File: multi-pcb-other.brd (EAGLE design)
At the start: 83.8 x 33 mm, 7 parts, among them X1 8B-ZR, X2 2.52B-ZR

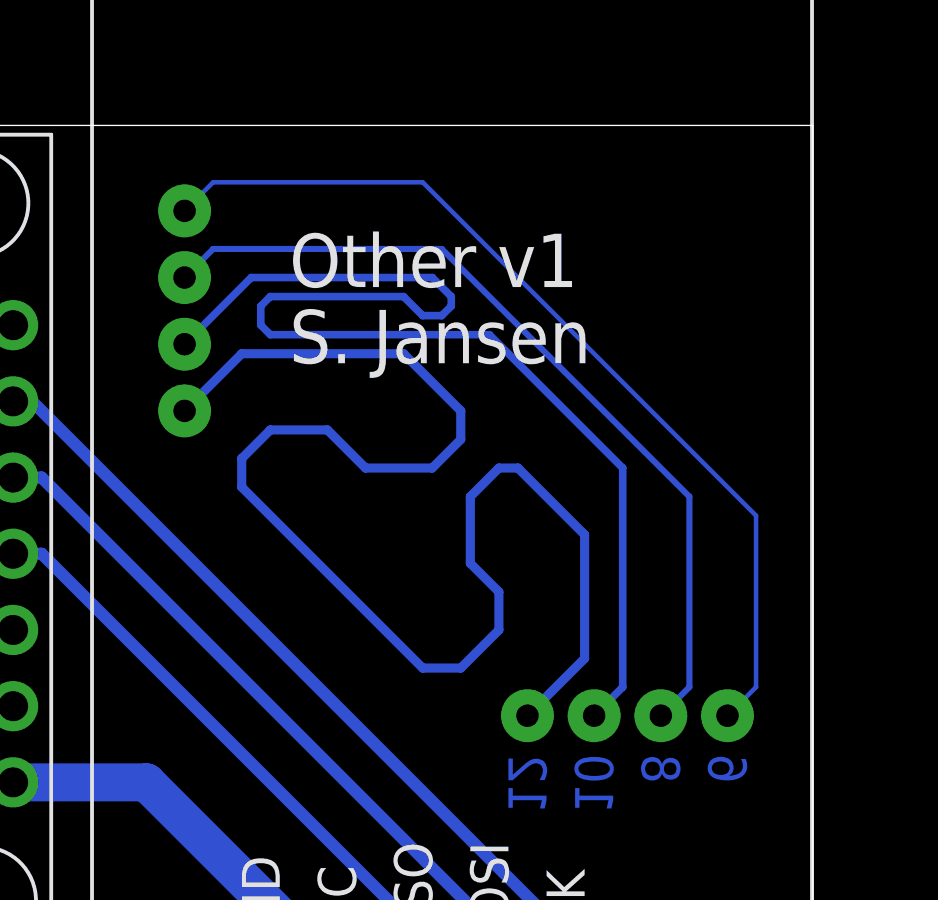
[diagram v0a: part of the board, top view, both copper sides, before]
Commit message: updated some PCB's
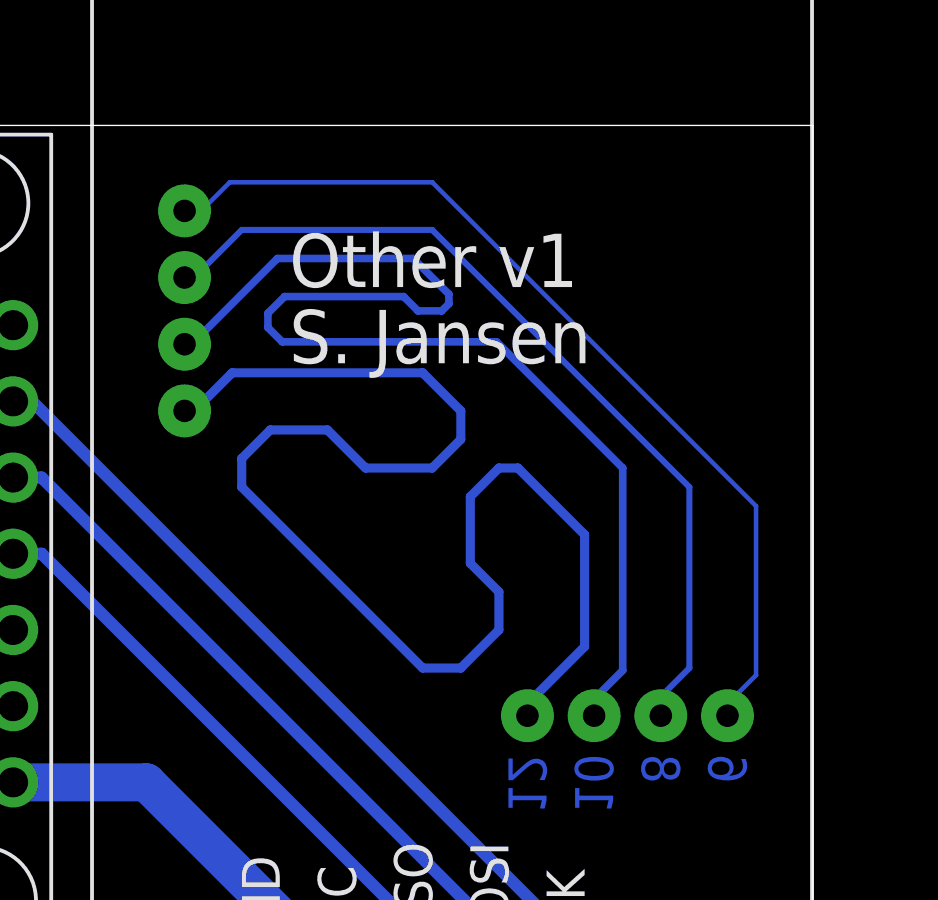
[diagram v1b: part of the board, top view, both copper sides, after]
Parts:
- R14: value 2k -> 1k
- R15: value 5k -> 2k
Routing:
- net N$2: track 28.3 -> 29.1 mm
- net N$4: track 49.7 -> 49.2 mm
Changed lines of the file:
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@@
 <setting verticaltext="up"/>
 </settings>
-<grid distance="12.5" unitdist="mil" unit="mil" style="lines" multiple="1" display="yes" altdistance="5" altunitdist="mil" altunit="mil"/>
+<grid distance="3.125" unitdist="mil" unit="mil" style="lines" multiple="1" display="yes" altdistance="5" altunitdist="mil" altunit="mil"/>
 <layers>
 <layer number="1" name="Top" color="4" fill="1" visible="yes" active="yes"/>
@@
 <attribute name="VALUE" x="37.1475" y="3.175" size="1.27" layer="27" rot="R90"/>
 </element>
-<element name="R14" library="rcl" library_urn="urn:adsk.eagle:library:334" package="0207/10" package3d_urn="urn:adsk.eagle:package:23491/2" value="2k" x="40.64" y="10.795" smashed="yes" rot="R270">
+<element name="R14" library="rcl" library_urn="urn:adsk.eagle:library:334" package="0207/10" package3d_urn="urn:adsk.eagle:package:23491/2" value="1k" x="40.64" y="10.795" smashed="yes" rot="R270">
 <attribute name="NAME" x="40.132" y="13.335" size="1.27" layer="25" ratio="10" rot="R270"/>
 <attribute name="POPULARITY" value="81" x="-26.67" y="-29.845" size="1.778" layer="27" rot="R270" display="off"/>
@@
 <attribute name="VALUE" x="40.0812" y="13.081" size="1.27" layer="27" ratio="10" rot="R270"/>
 </element>
-<element name="R15" library="rcl" library_urn="urn:adsk.eagle:library:334" package="0207/10" package3d_urn="urn:adsk.eagle:package:23491/2" value="5k" x="38.1" y="10.795" smashed="yes" rot="R270">
+<element name="R15" library="rcl" library_urn="urn:adsk.eagle:library:334" package="0207/10" package3d_urn="urn:adsk.eagle:package:23491/2" value="2k" x="38.1" y="10.795" smashed="yes" rot="R270">
 <attribute name="NAME" x="37.592" y="13.335" size="1.27" layer="25" ratio="10" rot="R270"/>
 <attribute name="POPULARITY" value="81" x="-29.21" y="-40.005" size="1.778" layer="27" rot="R270" display="off"/>
@@
 <contactref element="R15" pad="1"/>
 <contactref element="X1" pad="1"/>
-<polygon width="0.254" layer="16" spacing="0.1016" isolate="0.3048">
+<polygon width="0.254" layer="16" spacing="0.1016" isolate="0.3048" orphans="yes">
 <vertex x="-2.54" y="-2.2225"/>
 <vertex x="93.98" y="-2.2225"/>
@@
 <vertex x="-2.54" y="43.18"/>
 </polygon>
-<polygon width="0.1016" layer="16" spacing="0.1016" isolate="0.3048">
+<polygon width="0.1016" layer="16" spacing="0.1016" isolate="0.3048" orphans="yes">
 <vertex x="-1.27" y="-1.27"/>
 <vertex x="91.44" y="-1.27"/>
@@
 <signal name="N$1">
 <via x="62.865" y="25.7175" extent="1-16" drill="0.75"/>
-<wire x1="77.47" y1="14.2875" x2="76.5175" y2="13.335" width="0.254" layer="16"/>
+<wire x1="77.47" y1="14.843125" x2="76.5175" y2="13.890625" width="0.254" layer="16"/>
+<wire x1="76.5175" y1="13.890625" x2="76.5175" y2="13.335" width="0.254" layer="16"/>
 <via x="76.5175" y="13.335" extent="1-16" drill="0.75"/>
-<wire x1="71.12" y1="27.94" x2="71.755" y2="27.305" width="0.254" layer="16"/>
-<wire x1="71.755" y1="27.305" x2="71.755" y2="26.9875" width="0.254" layer="16"/>
-<wire x1="71.755" y1="26.9875" x2="71.4375" y2="26.67" width="0.254" layer="16"/>
-<wire x1="71.4375" y1="26.67" x2="70.8025" y2="26.67" width="0.254" layer="16"/>
-<wire x1="65.7225" y1="27.305" x2="65.405" y2="26.9875" width="0.254" layer="16"/>
-<wire x1="65.405" y1="26.9875" x2="65.405" y2="26.3525" width="0.254" layer="16"/>
-<wire x1="65.405" y1="26.3525" x2="65.7225" y2="26.035" width="0.254" layer="16"/>
-<wire x1="73.025" y1="26.035" x2="77.47" y2="21.59" width="0.254" layer="16"/>
-<wire x1="62.865" y1="25.7175" x2="65.0875" y2="27.94" width="0.254" layer="16"/>
-<wire x1="65.0875" y1="27.94" x2="71.12" y2="27.94" width="0.254" layer="16"/>
-<wire x1="70.8025" y1="26.67" x2="70.1675" y2="27.305" width="0.254" layer="16"/>
-<wire x1="70.1675" y1="27.305" x2="65.7225" y2="27.305" width="0.254" layer="16"/>
-<wire x1="65.7225" y1="26.035" x2="73.025" y2="26.035" width="0.254" layer="16"/>
-<wire x1="77.47" y1="21.59" x2="77.47" y2="14.2875" width="0.254" layer="16"/>
+<wire x1="70.485" y1="28.575" x2="71.675625" y2="27.384375" width="0.254" layer="16"/>
+<wire x1="71.675625" y1="27.384375" x2="71.675625" y2="27.066875" width="0.254" layer="16"/>
+<wire x1="71.675625" y1="27.066875" x2="71.4375" y2="26.82875" width="0.254" layer="16"/>
+<wire x1="71.4375" y1="26.82875" x2="70.64375" y2="26.82875" width="0.254" layer="16"/>
+<wire x1="66.19875" y1="27.305" x2="65.643125" y2="26.749375" width="0.254" layer="16"/>
+<wire x1="65.643125" y1="26.749375" x2="65.643125" y2="26.273125" width="0.254" layer="16"/>
+<wire x1="65.643125" y1="26.273125" x2="66.119375" y2="25.796875" width="0.254" layer="16"/>
+<wire x1="73.263125" y1="25.796875" x2="77.47" y2="21.59" width="0.254" layer="16"/>
+<wire x1="65.960625" y1="28.575" x2="63.103125" y2="25.7175" width="0.254" layer="16"/>
+<wire x1="62.865" y1="25.7175" x2="63.103125" y2="25.7175" width="0.254" layer="16"/>
+<wire x1="65.960625" y1="28.575" x2="70.485" y2="28.575" width="0.254" layer="16"/>
+<wire x1="70.64375" y1="26.82875" x2="70.1675" y2="27.305" width="0.254" layer="16"/>
+<wire x1="70.1675" y1="27.305" x2="66.19875" y2="27.305" width="0.254" layer="16"/>
+<wire x1="66.119375" y1="25.796875" x2="73.263125" y2="25.796875" width="0.254" layer="16"/>
+<wire x1="77.47" y1="21.59" x2="77.47" y2="14.843125" width="0.254" layer="16"/>
 </signal>
 <signal name="N$2">
 <via x="62.865" y="27.94" extent="1-16" drill="0.75"/>
-<wire x1="71.4375" y1="28.8925" x2="63.8175" y2="28.8925" width="0.2032" layer="16"/>
-<wire x1="62.865" y1="27.94" x2="63.8175" y2="28.8925" width="0.2032" layer="16"/>
-<wire x1="71.4375" y1="28.8925" x2="79.6925" y2="20.6375" width="0.2032" layer="16"/>
-<wire x1="79.6925" y1="20.6375" x2="79.6925" y2="14.2875" width="0.2032" layer="16"/>
-<wire x1="79.6925" y1="14.2875" x2="78.74" y2="13.335" width="0.2032" layer="16"/>
+<wire x1="71.12" y1="29.5275" x2="64.77" y2="29.5275" width="0.2032" layer="16"/>
+<wire x1="62.865" y1="27.94" x2="63.1825" y2="27.94" width="0.2032" layer="16"/>
+<wire x1="64.77" y1="29.5275" x2="63.1825" y2="27.94" width="0.2032" layer="16"/>
+<wire x1="71.12" y1="29.5275" x2="79.6925" y2="20.955" width="0.2032" layer="16"/>
+<wire x1="79.6925" y1="20.955" x2="79.6925" y2="14.9225" width="0.2032" layer="16"/>
+<wire x1="79.6925" y1="14.9225" x2="78.74" y2="13.97" width="0.2032" layer="16"/>
+<wire x1="78.74" y1="13.97" x2="78.74" y2="13.335" width="0.2032" layer="16"/>
 <via x="78.74" y="13.335" extent="1-16" drill="0.75"/>
 </signal>
@@
 <via x="62.865" y="30.1625" extent="1-16" drill="0.75"/>
 <via x="80.9625" y="13.335" extent="1-16" drill="0.75"/>
-<wire x1="62.865" y1="30.1625" x2="63.8175" y2="31.115" width="0.1524" layer="16"/>
-<wire x1="70.8025" y1="31.115" x2="81.915" y2="20.0025" width="0.1524" layer="16"/>
-<wire x1="81.915" y1="20.0025" x2="81.915" y2="14.2875" width="0.1524" layer="16"/>
-<wire x1="81.915" y1="14.2875" x2="80.9625" y2="13.335" width="0.1524" layer="16"/>
-<wire x1="63.8175" y1="31.115" x2="70.8025" y2="31.115" width="0.1524" layer="16"/>
+<wire x1="64.373125" y1="31.115" x2="63.420625" y2="30.1625" width="0.1524" layer="16"/>
+<wire x1="62.865" y1="30.1625" x2="63.420625" y2="30.1625" width="0.1524" layer="16"/>
+<wire x1="71.12" y1="31.115" x2="81.915" y2="20.32" width="0.1524" layer="16"/>
+<wire x1="81.915" y1="20.32" x2="81.915" y2="14.684375" width="0.1524" layer="16"/>
+<wire x1="81.915" y1="14.684375" x2="80.9625" y2="13.731875" width="0.1524" layer="16"/>
+<wire x1="80.9625" y1="13.731875" x2="80.9625" y2="13.335" width="0.1524" layer="16"/>
+<wire x1="64.373125" y1="31.115" x2="71.12" y2="31.115" width="0.1524" layer="16"/>
 </signal>
 <signal name="N$4">
 <via x="62.865" y="23.495" extent="1-16" drill="0.75"/>
-<wire x1="70.1675" y1="25.4" x2="64.77" y2="25.4" width="0.3048" layer="16"/>
-<wire x1="62.865" y1="23.495" x2="64.77" y2="25.4" width="0.3048" layer="16"/>
-<wire x1="76.2" y1="19.3675" x2="76.2" y2="15.24" width="0.3048" layer="16"/>
-<wire x1="76.2" y1="15.24" x2="74.295" y2="13.335" width="0.3048" layer="16"/>
+<wire x1="70.8025" y1="24.765" x2="64.4525" y2="24.765" width="0.3048" layer="16"/>
+<wire x1="64.4525" y1="24.765" x2="63.1825" y2="23.495" width="0.3048" layer="16"/>
+<wire x1="62.865" y1="23.495" x2="63.1825" y2="23.495" width="0.3048" layer="16"/>
+<wire x1="76.2" y1="19.3675" x2="76.2" y2="15.636875" width="0.3048" layer="16"/>
+<wire x1="76.2" y1="15.636875" x2="74.295" y2="13.731875" width="0.3048" layer="16"/>
+<wire x1="74.295" y1="13.731875" x2="74.295" y2="13.335" width="0.3048" layer="16"/>
 <via x="74.295" y="13.335" extent="1-16" drill="0.75"/>
-<wire x1="70.1675" y1="25.4" x2="72.0725" y2="23.495" width="0.3048" layer="16"/>
+<wire x1="70.8025" y1="24.765" x2="72.0725" y2="23.495" width="0.3048" layer="16"/>
 <wire x1="72.0725" y1="22.5425" x2="71.12" y2="21.59" width="0.3048" layer="16"/>
 <wire x1="71.12" y1="21.59" x2="68.8975" y2="21.59" width="0.3048" layer="16"/>
